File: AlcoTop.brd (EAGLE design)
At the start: 44.1 x 58.4 mm, 31 parts, among them IC4 ATMEGA328, Y1 16MHz

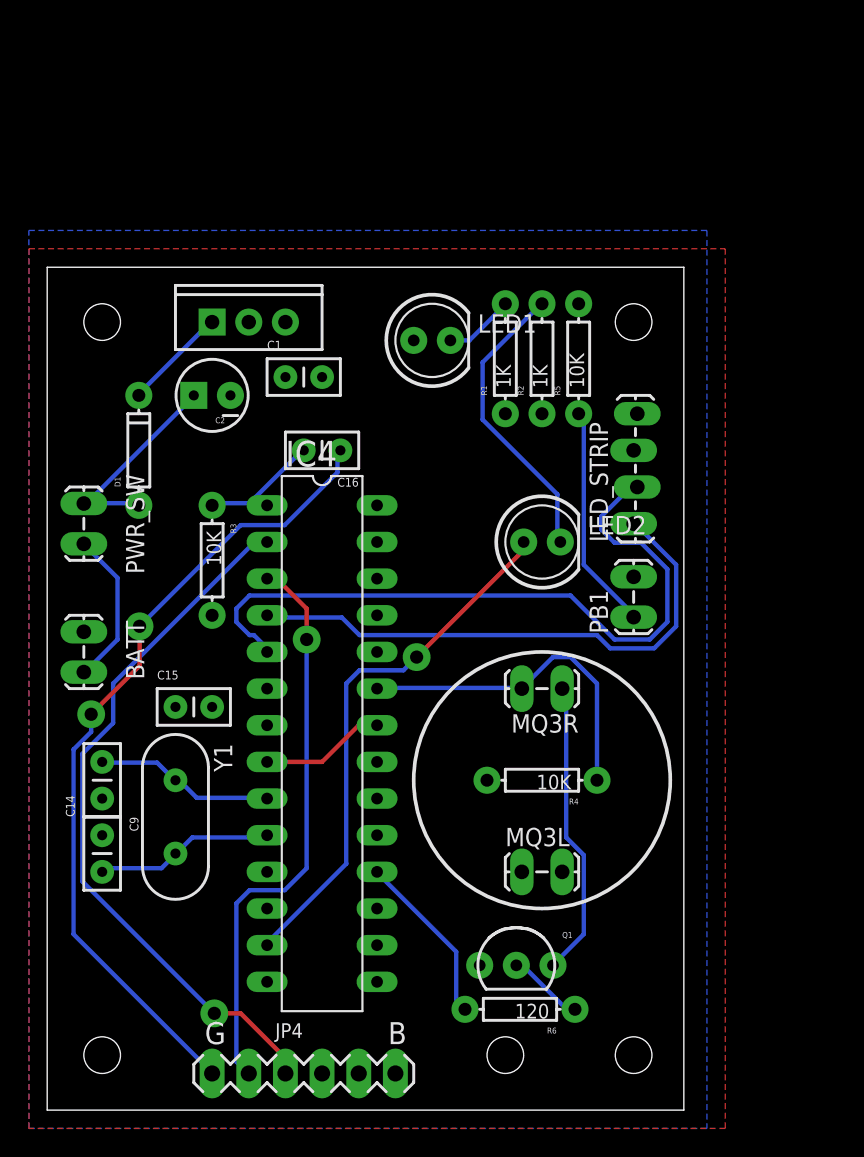
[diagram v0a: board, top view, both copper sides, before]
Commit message: Updated board
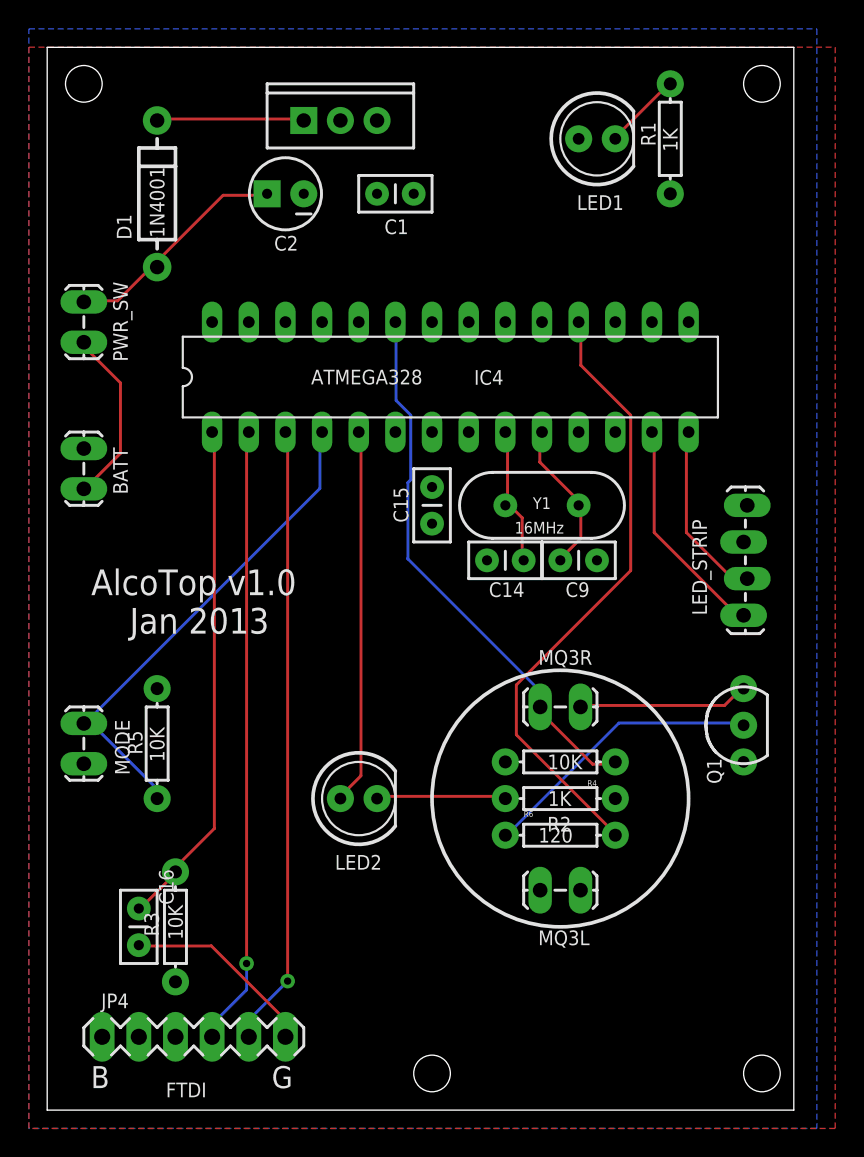
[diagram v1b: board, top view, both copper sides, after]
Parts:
- removed JP5: STAND-OFF#2, Dek:STAND-OFF-#2
- removed PB1: (no value), SparkFun-Connectors:1X02_LOCK_LONGPADS
- added MODE: (no value), Dek:1X02_LOCK_LONGPADS
- BATT, MQ3L, MQ3R, PWR_SW: device SparkFun-Connectors:1X02_LOCK_LONGPADS -> Dek:1X02_LOCK_LONGPADS
- D1: value (none) -> 1N4001; device Dek:DIODE-1N4148 -> Dek:DIODE-1N4001
- IC2: value (none) -> 7805; device SparkFun-PowerIC:TO220-IGO -> Dek:TO220-IGO
- IC4: device atmel:DIL28-3 -> Dek:DIL28-3
- LED1, LED2: device SparkFun-LED:LED5MM -> Dek:LED5MM
- LED_STRIP: device SparkFun-Connectors:1X04_LOCK_LONGPADS -> Dek:1X04_LOCK_LONGPADS
- Y1: device SparkFun:HC49US -> Dek:HC49US
- moved R5 39.6 mm to (7.62, 25.4)
- moved C9 39.2 mm to (38.1, 38.1), turned to 180 degrees
- moved C16 37.0 mm to (6.35, 11.4), turned to 90 degrees
- moved Y1 33.3 mm to (34.3, 41.9), turned to 0 degrees
- moved C14 31.4 mm to (30.5, 38.1), turned to 0 degrees
- moved R2 30.5 mm to (35.6, 21.6), turned to 180 degrees
- moved IC4 26.9 mm to (27.9, 50.8), turned to 0 degrees
- moved R3 25.5 mm to (8.89, 12.7)
- moved C15 23.4 mm to (26.7, 43.2), turned to 270 degrees
- moved Q1 22.9 mm to (48.3, 26.7), turned to 90 degrees
- moved LED2 21.8 mm to (21.6, 21.6)
- moved R1 19.1 mm to (43.2, 67.3)
- moved JP1 18.8 mm to (49.5, 71.1)
- moved LED1 18.1 mm to (38.1, 67.3)
- moved D1 17.8 mm to (7.62, 63.5)
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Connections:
- removed net SCL: PB1.1, R5.P$1
- net D2: now also MODE.1, R5.P$1; no longer LED_STRIP.1
- net D3: now also LED2.A; no longer LED_STRIP.2
- net D7: now also LED_STRIP.1; no longer LED2.A
- net D8: now also LED_STRIP.2
- net VCC: now also MODE.2; no longer PB1.2
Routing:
- net DTR: track 56.7 -> 13.5 mm, vias 2 -> 0
- net D12: track 12.1 -> 43.2 mm
- net RST: track 10.5 -> 35.5 mm
- net D3: track 49.8 -> 26.1 mm
- net D7: track 37.1 -> 15.6 mm, vias 1 -> 0
- net SCL: track 15.6 -> 0.00 mm
- net A0: track 23.7 -> 38.1 mm
- net N$7: track 5.42 -> 19.8 mm
- net D8: track 0.00 -> 12.6 mm
- net N$4: track 20.5 -> 9.08 mm
- net MQ3: track 20.7 -> 11.9 mm
- net GND: track 8.67 -> 0.00 mm
- net RX: track 49.6 -> 43.1 mm
- net D2: track 38.4 -> 34.9 mm
- net TX: track 39.8 -> 43.2 mm
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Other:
- board size 44.1 x 58.4 mm -> 51.7 x 73.7 mm
- board text added: "AlcoTop v1.0"
- board text added: "Jan 2013"
